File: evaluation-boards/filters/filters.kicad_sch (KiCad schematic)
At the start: 63 parts, among them J1 Conn_Coaxial, J10 Conn_Coaxial, J11 Conn_Coaxial, J12 Conn_Coaxial, J13 Conn_Coaxial, J14 Conn_Coaxial, J15 Conn_Coaxial, J16 Conn_Coaxial, J17 Conn_Coaxial, J18 Conn_Coaxial, J19 Conn_Coaxial, J2 Conn_Coaxial, J20 Conn_Coaxial, J3 Conn_Coaxial, J4 Conn_Coaxial, J5 Conn_Coaxial, J6 Conn_Coaxial, J7 Conn_Coaxial, J8 Conn_Coaxial, J9 Conn_Coaxial, U1 FIL-DEA, U3 FIL-LP0603, U5 5130BP18U4060, U7 2450HP

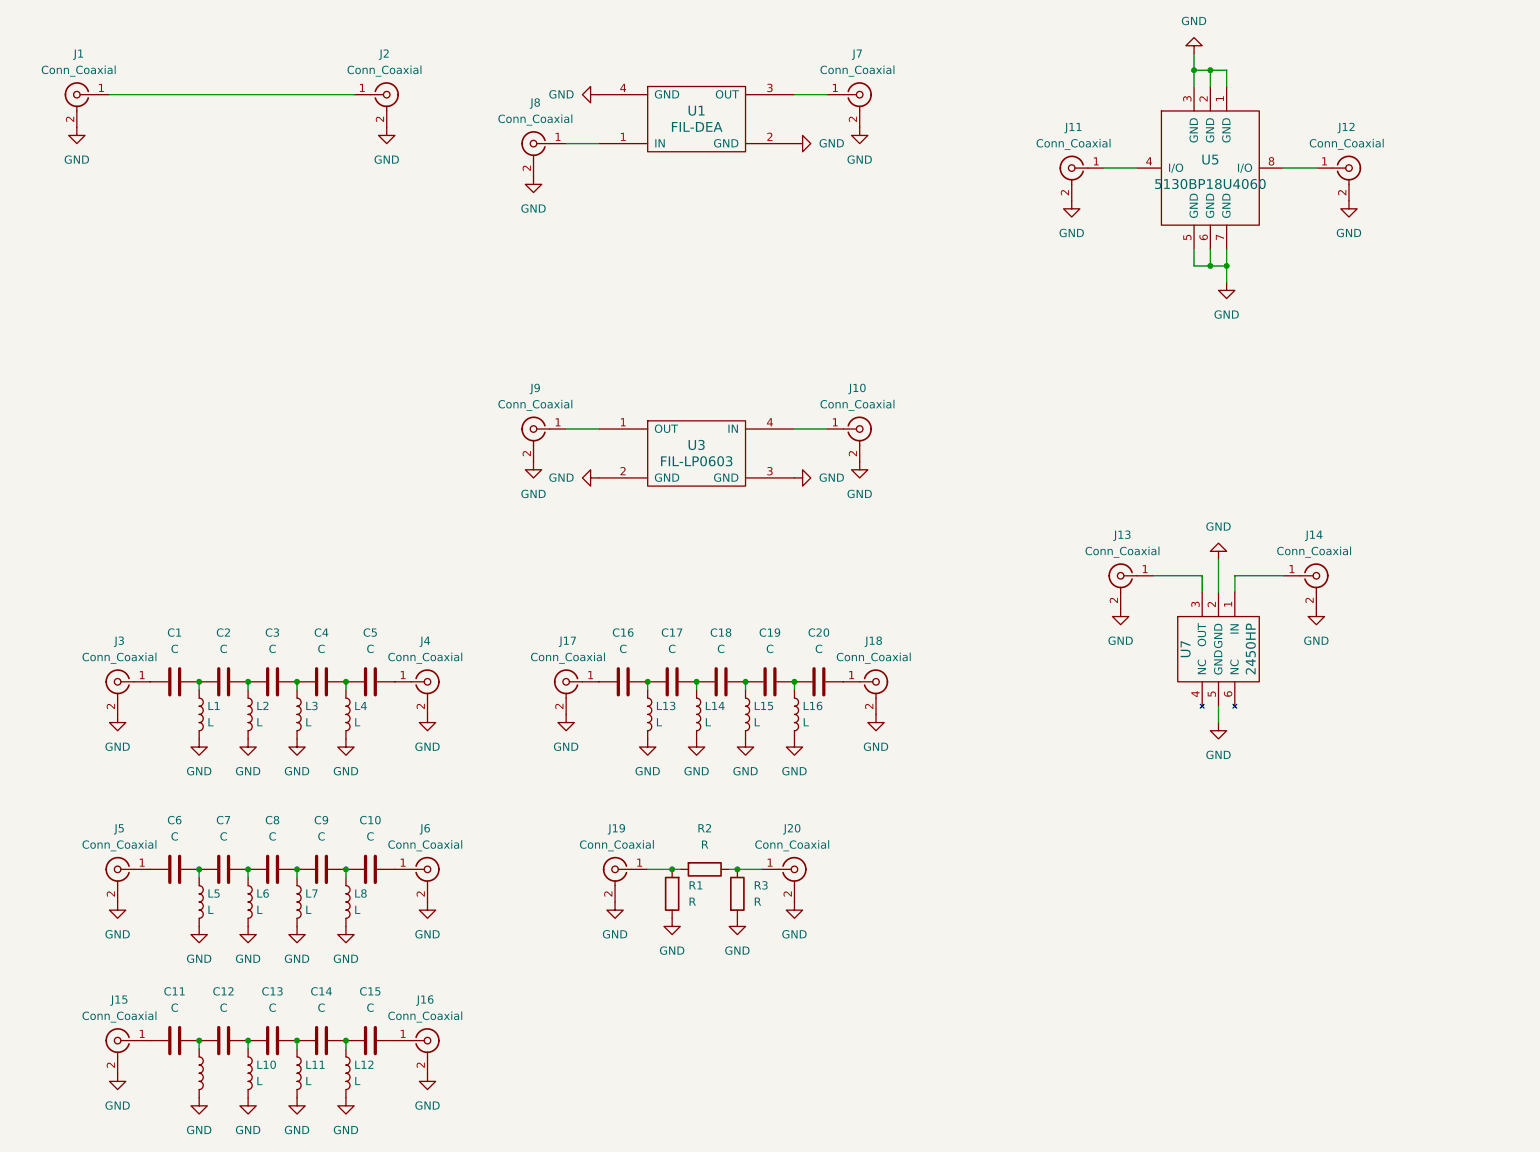
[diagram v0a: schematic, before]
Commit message: Update filters board
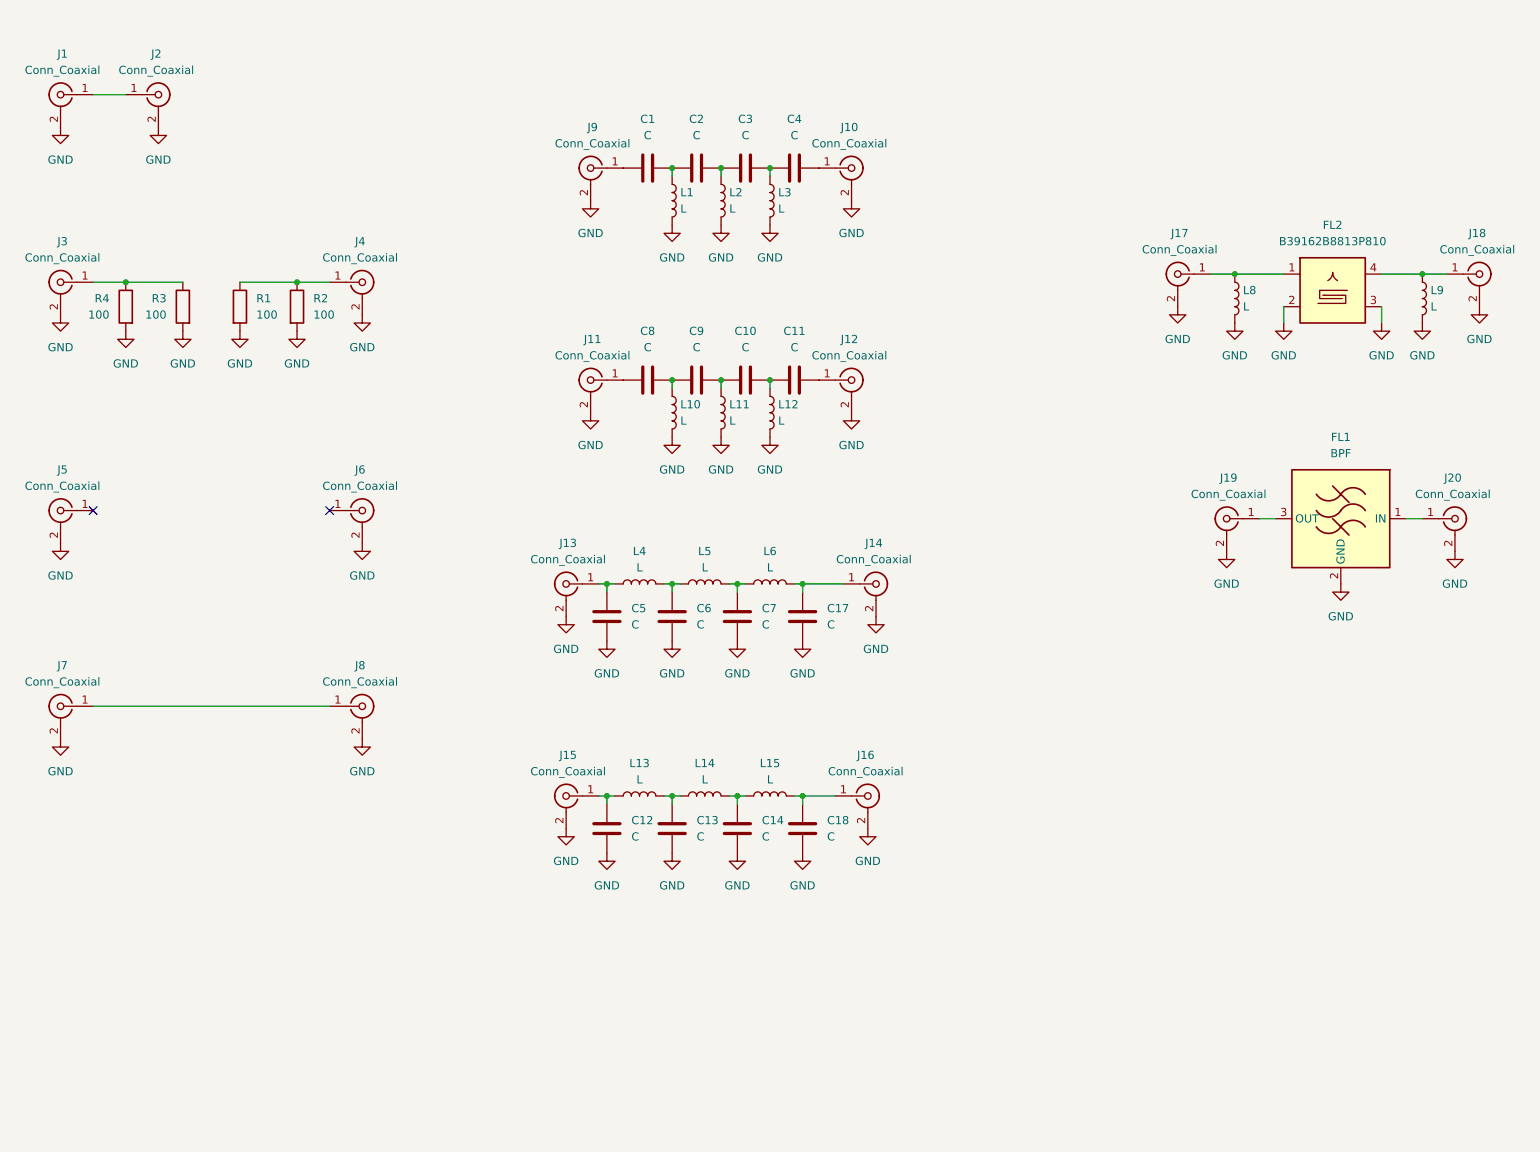
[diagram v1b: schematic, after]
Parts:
- removed C15, C16, C19, C20, C5: C, Capacitor_SMD:C_0201_0603Metric, symbol Device:C
- removed L16, L4, L7: L, Inductor_SMD:L_0201_0603Metric, symbol Device:L
- removed U1: FIL-DEA, gsg-modules:FIL-DEA-0603, symbol gsg-symbols:FIL-DEA
- removed U3: FIL-LP0603, gsg-modules:LP0603, symbol gsg-symbols:FIL-LP0603
- removed U5: 5130BP18U4060, gsg-modules:5130BP18U4060, symbol gsg-symbols:5130BP18U4060
- removed U7: 2450HP, gsg-modules:2500BL14M100, symbol gsg-symbols:2450HP
- added C8: C, Capacitor_SMD:C_0201_0603Metric, symbol Device:C
- added FL1: BPF, eval:Filter_Pulse_BPF1608LM09R5000A, symbol RF_Filter:BFCN-1445
- added FL2: B39162B8813P810, Filter:Filter_1109-5_1.1x0.9mm, symbol Filter:B39162B8813P810
- added L8: L, Inductor_SMD:L_0201_0603Metric, symbol Device:L
- added R4: 100, Resistor_SMD:R_0201_0603Metric, symbol Device:R
- R1, R2, R3: value R -> 100
- renumbered C8 to C5, L8 to L4
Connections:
- net GND: now also C12.1, C13.1, C14.1, C17.1, C18.1, C5.1, C6.1, C7.1, R1.2, R2.2, FL1.2 (GND), FL1.4 (GND), FL2.2, FL2.3, FL2.5, L8.2, R4.2; no longer L13.2, L14.2, L15.2, L4.2, L5.2, L6.2, R1.1
- net at J8.1 (In): now also J7.1 (In)
- net at J9.1 (In): now also C1.1
- net at J10.1 (In): now also C4.2
- net at J11.1 (In): now also C8.1
- net at J12.1 (In): now also C11.2
- net at J14.1 (In): now also C17.2, L6.2
- net at J13.1 (In): now also C5.2, L4.1
- net at J4.1 (In): now also R1.1, R2.1
- net at J16.1 (In): now also C18.2, L15.2
- net at C9.1: now also L10.1, C8.2; no longer C5.2
- net at J18.1 (In): now also L9.1, FL2.4
- net at L15.1: now also C14.2, L14.2; no longer C18.2
- net at L12.1: now also C10.2, C11.1; no longer C14.2
- net at J3.1 (In): now also R3.1, R4.1; no longer C1.1
- net at L13.1: now also C12.2, J15.1 (In); no longer C17.1
- net at C6.2, L5.1: now also L4.2; no longer C7.1
- net at C7.2, L6.1: now also L5.2; no longer C5.1
- net at C10.1, C9.2: now also L11.1; no longer L4.1
- net at J17.1 (In): now also FL2.1, L8.1
- net at J5.1 (In): no longer C6.1
- net at J6.1 (In): no longer C10.2
- new net: FL1.1 (IN), J20.1 (In)
- new net: FL1.3 (OUT), J19.1 (In)
- new net: C13.2, L13.2, L14.1
- no-connect marks 0 -> 2
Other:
- moved on the sheet: C1, C2, C3, C4, C5, C6, C7, J1, J2, J3, J4, J5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
